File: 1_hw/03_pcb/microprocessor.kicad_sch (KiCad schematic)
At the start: 29 parts, among them SW1 TS-1187A-B-A-B, SW2 SS-12D02-VG4, SW3 SS-12D02-VG4, U11 STM32F446ZETx, Y1 32.768k

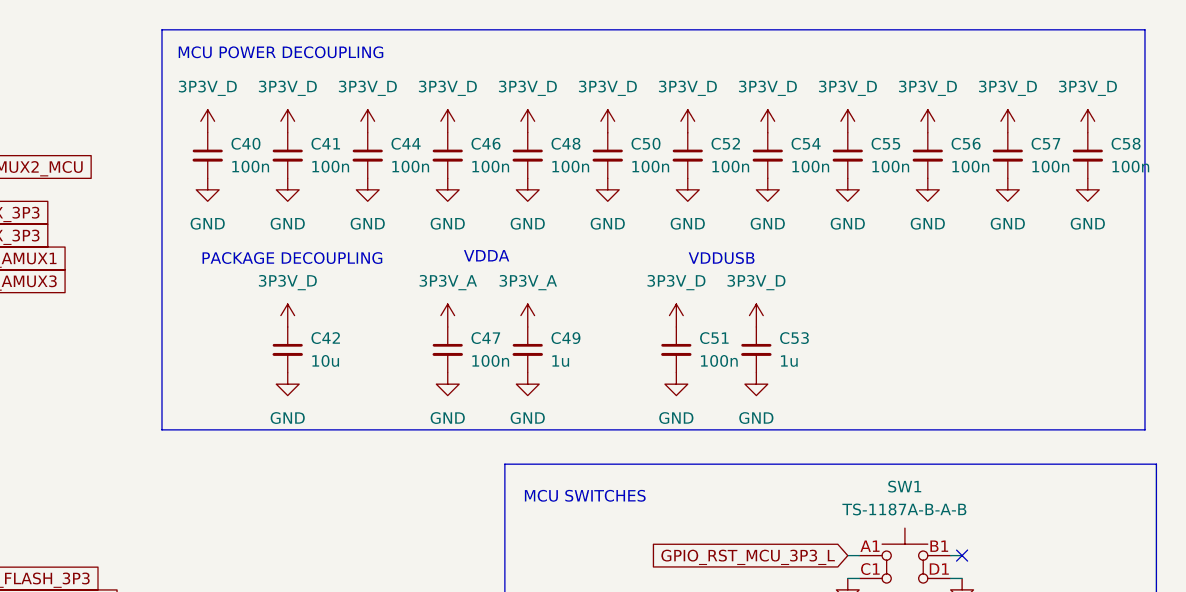
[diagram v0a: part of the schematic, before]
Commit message: FEAT: Finished placement of components, switches, etc.
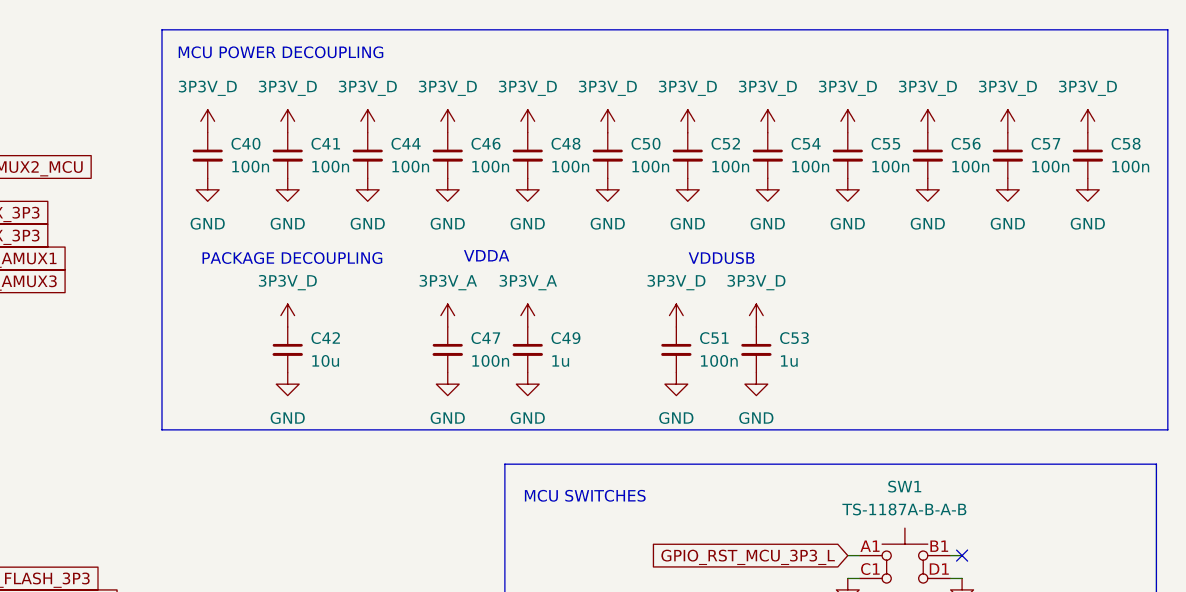
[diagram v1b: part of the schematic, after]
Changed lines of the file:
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@@
 	(rectangle
 		(start 149.86 13.97)
-		(end 259.08 58.42)
+		(end 261.62 58.42)
 		(stroke
 			(width 0)
